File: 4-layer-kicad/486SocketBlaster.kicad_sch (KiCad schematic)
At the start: 18 parts, among them U1 TPS563200

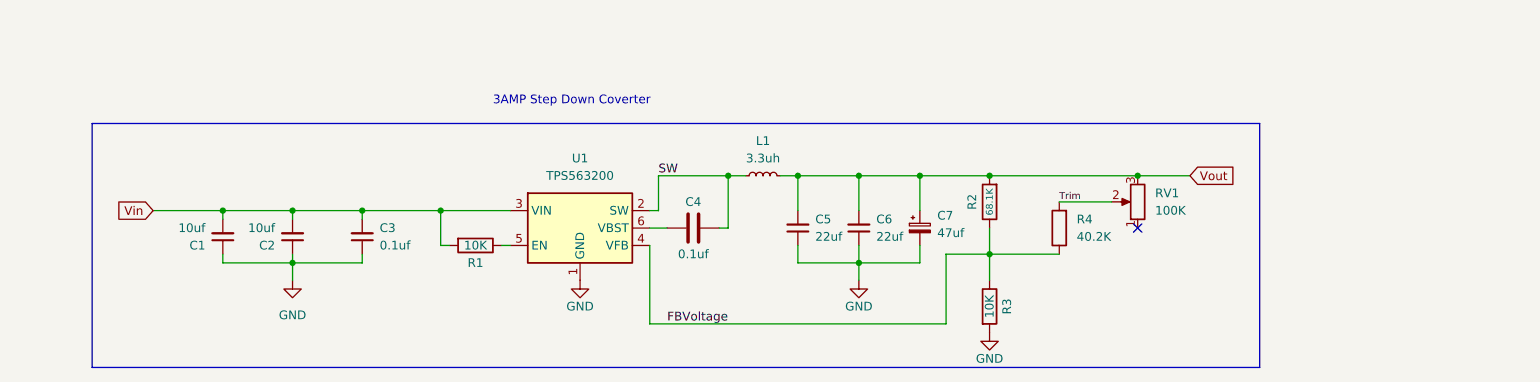
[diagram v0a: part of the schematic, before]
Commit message: update
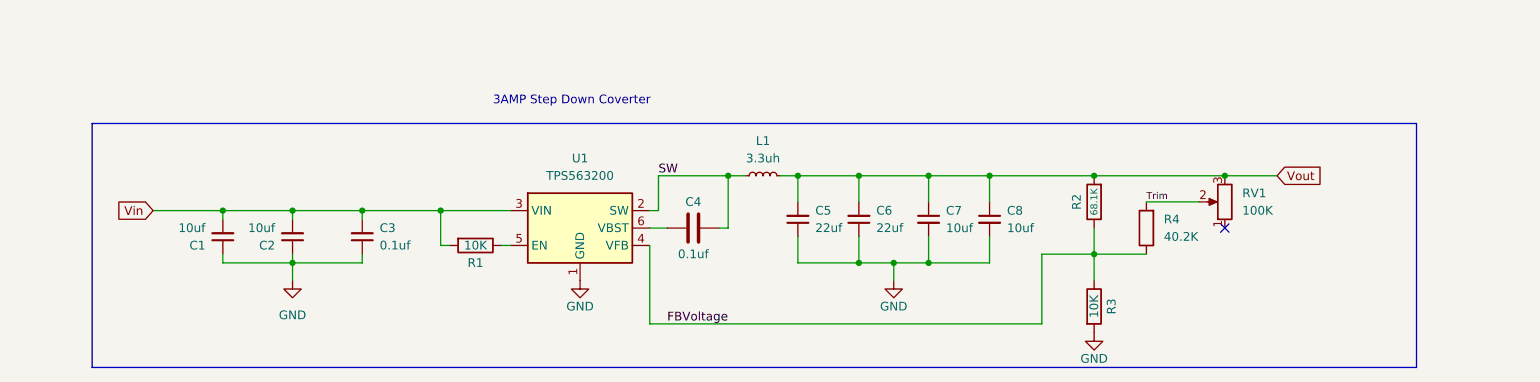
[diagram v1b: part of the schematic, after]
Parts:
- removed C7: 47uf, 486SocketBlaster:CP_EIA-3216-12_Kemet-S_Pad1.58x1.35mm_HandSolder, symbol Device:C_Polarized_Small
- added C7, C8: 10uf, 486SocketBlaster:C_0805_2012Metric, symbol Device:C_Small
- C3, C4: footprint 486SocketBlaster:C_0603_1608Metric -> 486SocketBlaster:C_0805_2012Metric
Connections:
- net GND: now also C7.2, C8.2
- net Vout: now also C7.1, C8.1
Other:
- moved on the sheet: C5, C6, R2, R3, R4, RV1
